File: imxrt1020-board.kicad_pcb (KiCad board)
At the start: 2 copper layers, 102.9 x 68.6 mm, 200 parts, among them J1 Micro_SD_Card_Det, J10 CASTELATED, J11 CASTELATED, J12 CASTELATED, J13 CASTELATED, J14 CASTELATED, J15 CASTELATED, J16 CASTELATED, J17 CASTELATED, J18 CASTELATED, J19 CASTELATED, J2 USB_OTG, J20 CASTELATED, J21 CASTELATED, J22 CASTELATED, J23 CASTELATED, J24 CASTELATED, J25 CASTELATED, J26 CASTELATED, J27 CASTELATED, J28 CASTELATED, J29 CASTELATED, J3 Conn_02x20_Odd_Even, J30 CASTELATED, J31 CASTELATED, J32 CASTELATED, J33 CASTELATED, J34 CASTELATED, J35 CASTELATED, J36 CASTELATED, J37 CASTELATED, J38 CASTELATED, J39 CASTELATED, J4 CASTELATED, J40 CASTELATED, J41 CASTELATED, J42 CASTELATED, J43 CASTELATED, J44 GS2, J45 GS2, J46 PWR_IN, J47 JTAG, J48 Conn_01x06, J49 CASTELATED, J5 CASTELATED, J50 CASTELATED, J51 CASTELATED, J52 CASTELATED, J53 CASTELATED, J54 CASTELATED, J55 CASTELATED, J56 CASTELATED, J57 CASTELATED, J58 SI-50196-F, J59 CASTELATED, J6 CASTELATED, J60 CASTELATED, J61 CASTELATED, J62 CASTELATED, J63 CASTELATED, J64 CASTELATED, J65 CASTELATED, J66 CASTELATED, J67 CASTELATED, J68 CASTELATED, J69 CASTELATED, J7 CASTELATED, J70 CASTELATED, J71 CASTELATED, J72 CASTELATED, J73 CASTELATED, J74 CASTELATED, J75 CASTELATED, J76 CASTELATED, J77 CASTELATED, J78 CASTELATED, J79 CASTELATED, J8 CASTELATED, J80 CASTELATED, J81 Conn_01x07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

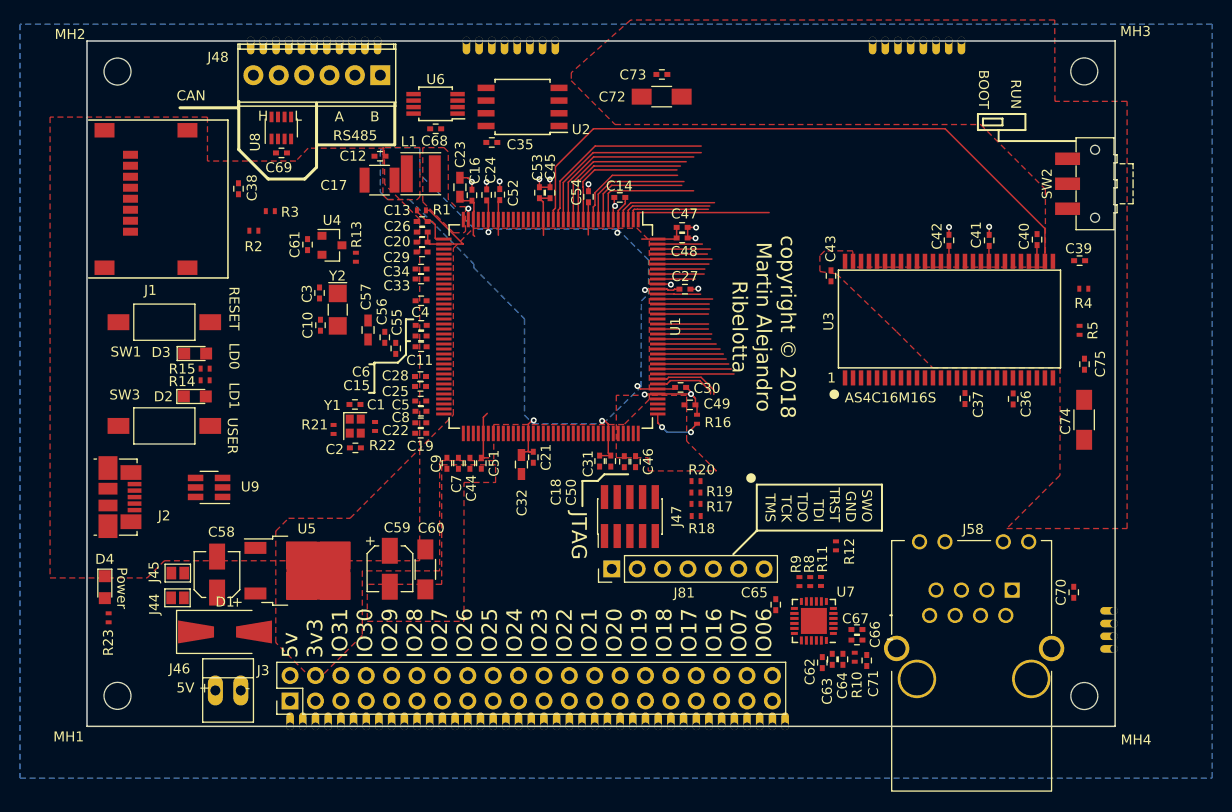
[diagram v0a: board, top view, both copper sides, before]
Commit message: Save commit after kicad-5 migration
Signed-off-by: Martin Ribelotta <martinribelotta@gmail.com>
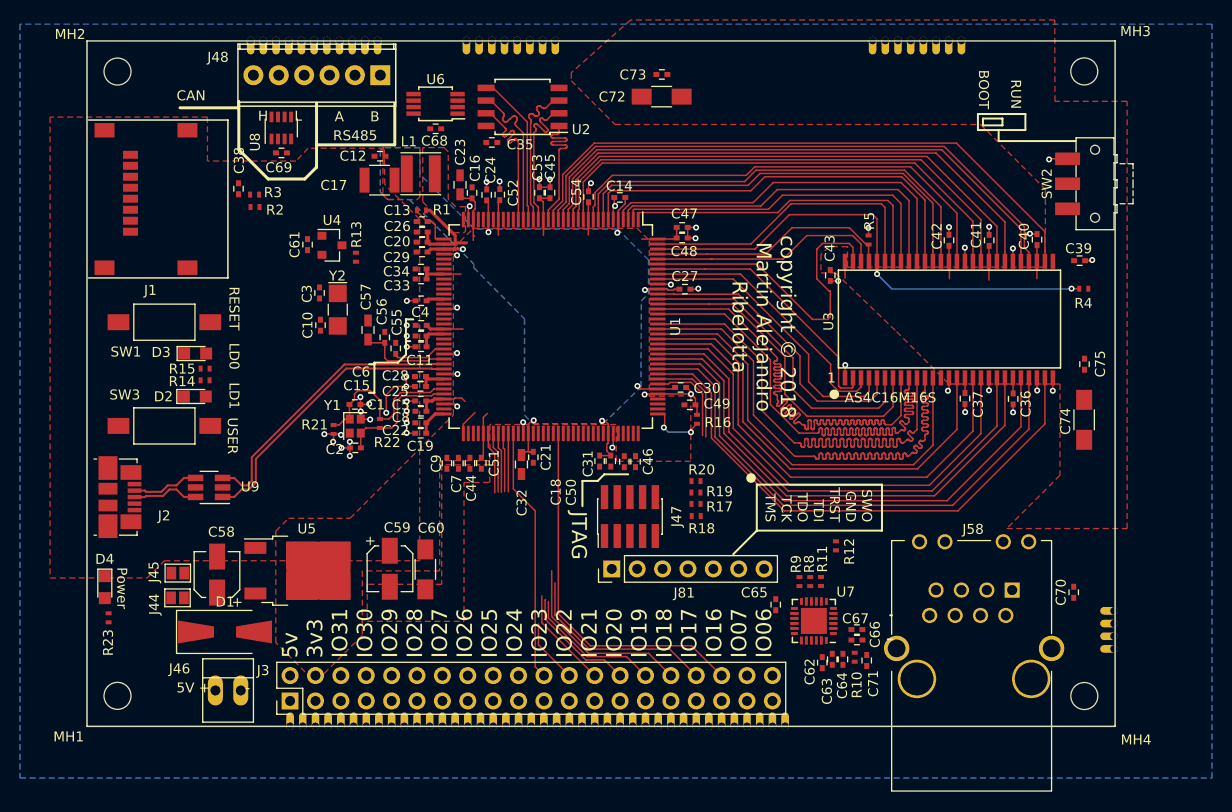
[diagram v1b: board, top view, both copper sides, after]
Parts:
- moved R5 23.0 mm to (186.0, 91.2), turned to 90 degrees
- moved R2 2.38 mm to (124.6, 87.9), turned to 0 degrees
- moved R3 2.28 mm to (124.5, 86.6), turned to 0 degrees
- moved R22 0.57 mm to (137.1, 109.5)
- moved C16 0.24 mm to (146.3, 86.4)
- moved C23 0.24 mm to (145.1, 85.6)
- moved C43 0.08 mm to (182.1, 94.7)
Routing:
- net /MEMORY/SDRAM_CLK: track 5.07 -> 61.2 mm
- net /MEMORY/SDRAM_A12: track 5.08 -> 61.1 mm
- net /MEMORY/SDRAM_CKE: track 5.08 -> 61.1 mm
- net /MEMORY/SDRAM_A11: track 5.15 -> 61.1 mm
- net /MEMORY/SDRAM_Q15: track 7.63 -> 55.3 mm
- net /MEMORY/SDRAM_Q14: track 7.36 -> 54.0 mm
- net /MEMORY/SDRAM_Q13: track 7.10 -> 53.1 mm
- net /MEMORY/SDRAM_A0: track 5.27 -> 49.9 mm, vias 0 -> 2
- net /MEMORY/SDRAM_Q12: track 6.85 -> 51.2 mm
- net GND: track 24.8 -> 69.0 mm, vias 16 -> 57
- net /MEMORY/SDRAM_Q11: track 6.56 -> 50.2 mm
- net /MEMORY/SDRAM_Q10: track 6.24 -> 48.9 mm
- net /MEMORY/SDRAM_Q9: track 5.85 -> 47.4 mm
- net /MEMORY/SDRAM_Q8: track 5.31 -> 45.3 mm
- net /MEMORY/SDRAM_Q1: track 19.5 -> 58.7 mm
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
